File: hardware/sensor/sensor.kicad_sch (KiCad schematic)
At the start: 10 parts

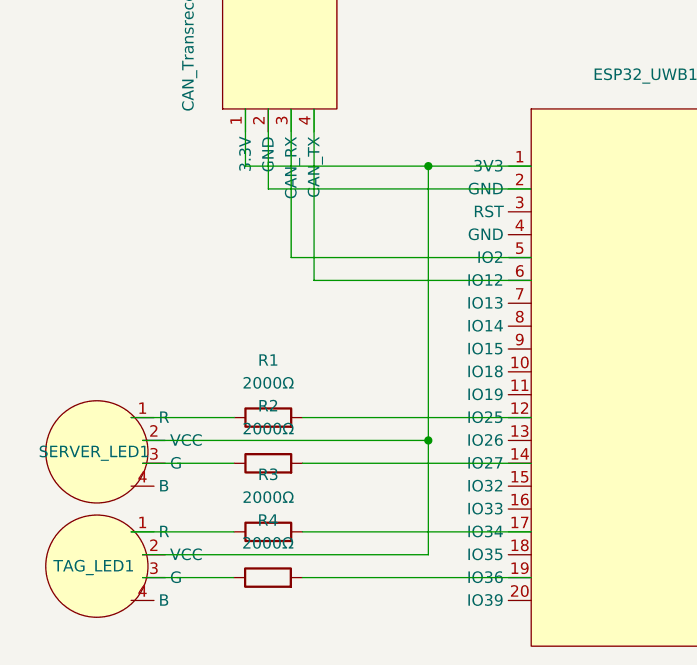
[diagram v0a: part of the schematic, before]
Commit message: hardware: Add remote PCB.
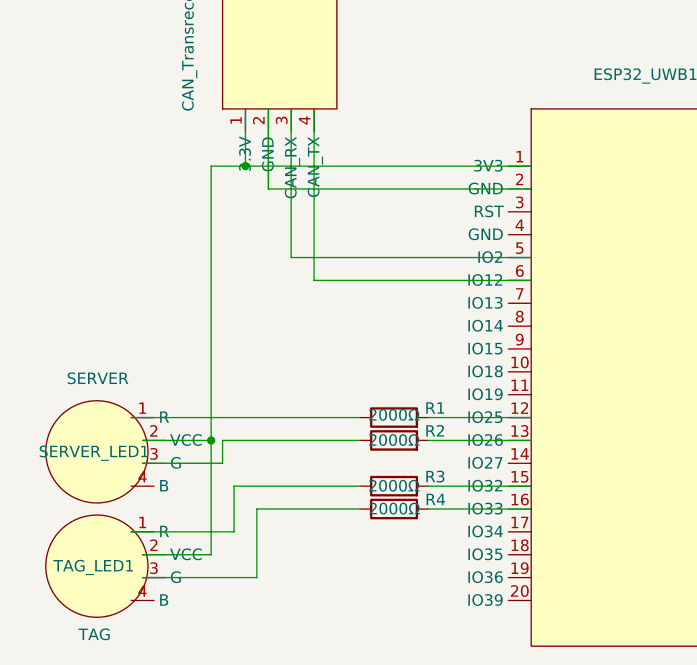
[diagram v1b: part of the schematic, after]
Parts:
- SERVER_LED1: value ~ -> SERVER
- TAG_LED1: value ~ -> TAG
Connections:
- net at R3.2: now also ESP32_UWB1.15 (IO32); no longer ESP32_UWB1.17 (IO34)
- net at R4.2: now also ESP32_UWB1.16 (IO33); no longer ESP32_UWB1.19 (IO36)
- net at ESP32_UWB1.13 (IO26): now also R2.2
- net at ESP32_UWB1.14 (IO27): no longer R2.2
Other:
- moved on the sheet: R1, R2, R3, R4
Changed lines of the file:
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@@
 	)
 	(junction
-		(at 125.73 120.65)
+		(at 105.41 90.17)
 		(diameter 0)
 		(color 0 0 0 0)
 	)
 	(junction
-		(at 125.73 90.17)
+		(at 101.6 120.65)
 		(diameter 0)
 		(color 0 0 0 0)
@@
 	(wire
 		(pts
-			(xy 93.98 120.65) (xy 125.73 120.65)
-		)
-		(stroke
-			(width 0)
-			(type default)
-		)
-	)
-	(wire
-		(pts
-			(xy 125.73 90.17) (xy 125.73 120.65)
+			(xy 93.98 120.65) (xy 101.6 120.65)
+		)
+		(stroke
+			(width 0)
+			(type default)
+		)
+	)
+	(wire
+		(pts
+			(xy 101.6 90.17) (xy 101.6 120.65)
 		)
 		(stroke
@@
 	(wire
 		(pts
-			(xy 125.73 90.17) (xy 137.16 90.17)
+			(xy 104.14 125.73) (xy 104.14 130.81)
 		)
 		(stroke
@@
 	(wire
 		(pts
-			(xy 92.71 130.81) (xy 104.14 130.81)
-		)
-		(stroke
-			(width 0)
-			(type default)
-		)
-	)
-	(wire
-		(pts
 			(xy 110.49 100.33) (xy 137.16 100.33)
 		)
@@
 	(wire
 		(pts
-			(xy 93.98 133.35) (xy 125.73 133.35)
-		)
-		(stroke
-			(width 0)
-			(type default)
-		)
-	)
-	(wire
-		(pts
-			(xy 111.76 123.19) (xy 137.16 123.19)
+			(xy 93.98 133.35) (xy 101.6 133.35)
 		)
 		(stroke
@@
 	(wire
 		(pts
-			(xy 111.7236 135.89) (xy 137.16 135.89)
+			(xy 106.68 128.27) (xy 106.68 135.89)
+		)
+		(stroke
+			(width 0)
+			(type default)
+		)
+	)
+	(wire
+		(pts
+			(xy 104.14 130.81) (xy 92.71 130.81)
+		)
+		(stroke
+			(width 0)
+			(type default)
+		)
+	)
+	(wire
+		(pts
+			(xy 105.41 90.17) (xy 137.16 90.17)
+		)
+		(stroke
+			(width 0)
+			(type default)
+		)
+	)
+	(wire
+		(pts
+			(xy 101.6 90.17) (xy 105.41 90.17)
 		)
 		(stroke
@@
 	(wire
 		(pts
-			(xy 111.76 118.11) (xy 137.16 118.11)
+			(xy 125.73 128.27) (xy 137.16 128.27)
+		)
+		(stroke
+			(width 0)
+			(type default)
+		)
+	)
+	(wire
+		(pts
+			(xy 125.73 120.65) (xy 137.16 120.65)
+		)
+		(stroke
+			(width 0)
+			(type default)
+		)
+	)
+	(wire
+		(pts
+			(xy 125.73 125.73) (xy 137.16 125.73)
+		)
+		(stroke
+			(width 0)
+			(type default)
+		)
+	)
+	(wire
+		(pts
+			(xy 125.73 118.11) (xy 137.16 118.11)
 		)
 		(stroke
@@
 	(wire
 		(pts
+			(xy 118.11 128.27) (xy 106.68 128.27)
+		)
+		(stroke
+			(width 0)
+			(type default)
+		)
+	)
+	(wire
+		(pts
+			(xy 102.87 120.65) (xy 102.87 123.19)
+		)
+		(stroke
+			(width 0)
+			(type default)
+		)
+	)
+	(wire
+		(pts
 			(xy 113.03 83.82) (xy 113.03 102.87)
 		)
@@
 	(wire
 		(pts
-			(xy 93.98 135.89) (xy 104.1036 135.89)
-		)
-		(stroke
-			(width 0)
-			(type default)
-		)
-	)
-	(wire
-		(pts
 			(xy 213.36 101.6) (xy 213.36 92.71)
 		)
@@
 	(wire
 		(pts
-			(xy 111.76 130.81) (xy 137.16 130.81)
-		)
-		(stroke
-			(width 0)
-			(type default)
-		)
-	)
-	(wire
-		(pts
-			(xy 105.41 90.17) (xy 125.73 90.17)
+			(xy 118.11 125.73) (xy 104.14 125.73)
 		)
 		(stroke
@@
 	(wire
 		(pts
-			(xy 92.71 118.11) (xy 104.14 118.11)
-		)
-		(stroke
-			(width 0)
-			(type default)
-		)
-	)
-	(wire
-		(pts
-			(xy 125.73 120.65) (xy 125.73 133.35)
-		)
-		(stroke
-			(width 0)
-			(type default)
-		)
-	)
-	(wire
-		(pts
-			(xy 93.98 123.19) (xy 104.14 123.19)
+			(xy 92.71 118.11) (xy 118.11 118.11)
+		)
+		(stroke
+			(width 0)
+			(type default)
+		)
+	)
+	(wire
+		(pts
+			(xy 101.6 120.65) (xy 101.6 133.35)
+		)
+		(stroke
+			(width 0)
+			(type default)
+		)
+	)
+	(wire
+		(pts
+			(xy 106.68 135.89) (xy 93.98 135.89)
+		)
+		(stroke
+			(width 0)
+			(type default)
+		)
+	)
+	(wire
+		(pts
+			(xy 102.87 120.65) (xy 118.11 120.65)
 		)
 		(stroke
@@
 		(pts
 			(xy 162.56 90.17) (xy 181.61 90.17)
+		)
+		(stroke
+			(width 0)
+			(type default)
+		)
+	)
+	(wire
+		(pts
+			(xy 102.87 123.19) (xy 93.98 123.19)
 		)
 		(stroke
@@
 	(symbol
 		(lib_id "Autocam:Simple Resistor")
-		(at 107.95 130.81 90)
+		(at 121.92 125.73 90)
 		(unit 1)
 		(exclude_from_sim no)
@@
 		(dnp no)
 		(property "Reference" "R3"
-			(at 107.95 124.46 90)
+			(at 126.492 124.714 90)
 			(effects
 				(font
@@
 		)
 		(property "Value" "2000Ω"
-			(at 107.95 127 90)
+			(at 121.92 125.73 90)
 			(effects
 				(font
@@
 		)
 		(property "Footprint" "Autocam:Simple Resistor"
-			(at 107.95 132.588 90)
+			(at 121.92 127.508 90)
 			(effects
 				(font
@@
 		)
 		(property "Datasheet" "~"
-			(at 107.95 130.81 0)
+			(at 121.92 125.73 0)
 			(effects
 				(font
@@
 		)
 		(property "Description" "Resistor"
-			(at 107.95 130.81 0)
+			(at 121.92 125.73 0)
 			(effects
 				(font
@@
 			)
 		)
-		(property "Value" "~"
-			(at 97.79 133.35 90)
+		(property "Value" "TAG"
+			(at 86.868 142.24 90)
 			(effects
 				(font
@@
 			)
 		)
-		(property "Value" "~"
-			(at 91.1402 128.27 0)
+		(property "Value" "SERVER"
+			(at 92.456 113.792 90)
 			(effects
 				(font
@@
 	(symbol
 		(lib_id "Autocam:Simple Resistor")
-		(at 107.9136 135.89 90)
+		(at 121.92 128.27 90)
 		(unit 1)
 		(exclude_from_sim no)
@@
 		(dnp no)
 		(property "Reference" "R4"
-			(at 107.9136 129.54 90)
+			(at 126.5284 127.254 90)
 			(effects
 				(font
@@
 		)
 		(property "Value" "2000Ω"
-			(at 107.9136 132.08 90)
+			(at 121.9564 128.27 90)
 			(effects
 				(font
@@
 		)
 		(property "Footprint" "Autocam:Simple Resistor"
-			(at 107.9136 137.668 90)
+			(at 121.92 130.048 90)
 			(effects
 				(font
@@
 		)
 		(property "Datasheet" "~"
-			(at 107.9136 135.89 0)
+			(at 121.92 128.27 0)
 			(effects
 				(font
@@
 		)
 		(property "Description" "Resistor"
-			(at 107.9136 135.89 0)
+			(at 121.92 128.27 0)
 			(effects
 				(font
@@
 	(symbol
 		(lib_id "Autocam:Simple Resistor")
-		(at 107.95 118.11 90)
+		(at 121.92 118.11 90)
 		(unit 1)
 		(exclude_from_sim no)
@@
 		(dnp no)
 		(property "Reference" "R1"
-			(at 107.95 111.76 90)
+			(at 126.492 117.094 90)
 			(effects
 				(font
@@
 		)
 		(property "Value" "2000Ω"
-			(at 107.95 114.3 90)
+			(at 121.92 117.856 90)
 			(effects
 				(font
@@
 		)
 		(property "Footprint" "Autocam:Simple Resistor"
-			(at 107.95 119.888 90)
+			(at 121.92 119.888 90)
 			(effects
 				(font
@@
 		)
 		(property "Datasheet" "~"
-			(at 107.95 118.11 0)
+			(at 121.92 118.11 0)
 			(effects
 				(font
@@
 		)
 		(property "Description" "Resistor"
-			(at 107.95 118.11 0)
+			(at 121.92 118.11 0)
 			(effects
 				(font
@@
 	(symbol
 		(lib_id "Autocam:Simple Resistor")
-		(at 107.95 123.19 90)
+		(at 121.92 120.65 90)
 		(unit 1)
 		(exclude_from_sim no)
@@
 		(dnp no)
 		(property "Reference" "R2"
-			(at 107.95 116.84 90)
+			(at 126.492 119.634 90)
 			(effects
 				(font
@@
 		)
 		(property "Value" "2000Ω"
-			(at 107.95 119.38 90)
+			(at 121.92 120.65 90)
 			(effects
 				(font
@@
 		)
 		(property "Footprint" "Autocam:Simple Resistor"
-			(at 107.95 124.968 90)
+			(at 121.92 122.428 90)
 			(effects
 				(font
@@
 		)
 		(property "Datasheet" "~"
-			(at 107.95 123.19 0)
+			(at 121.92 120.65 0)
 			(effects
 				(font
@@
 		)
 		(property "Description" "Resistor"
-			(at 107.95 123.19 0)
-			(effects
-				(font
+			(at 121.92 120.65 0)
+			(effects
+				(font
